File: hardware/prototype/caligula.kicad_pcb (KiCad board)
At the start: 2 copper layers, 89.8 x 108.2 mm, 105 parts, among them J1 USB2UART, J10 PT100_CONN, J2 1.47 IPS LCD, J3 ConnBattery, J4 USB2UART, J5 lcd jumper, J6 lcd jumper, J7 lcd jumper, J8 PH Sensor, Q1 SS8050, Q2 SS8050, Q3 SS8050, SW1 RST, SW2 IN1, SW3 Boot, SW4 IN2, SW5 IN4, SW6 IN4, SW7 MST22D18G2, U1 CH340C, U2 ESP32-S3-WROOM-1, U3 TPS63001_SEPIC_3V3, U4 ICL7660, U5 BQ24075RGT_DPPM, U6 ADS1115IDGS, U7 MAX31865xTP, U8 OPA2197xD

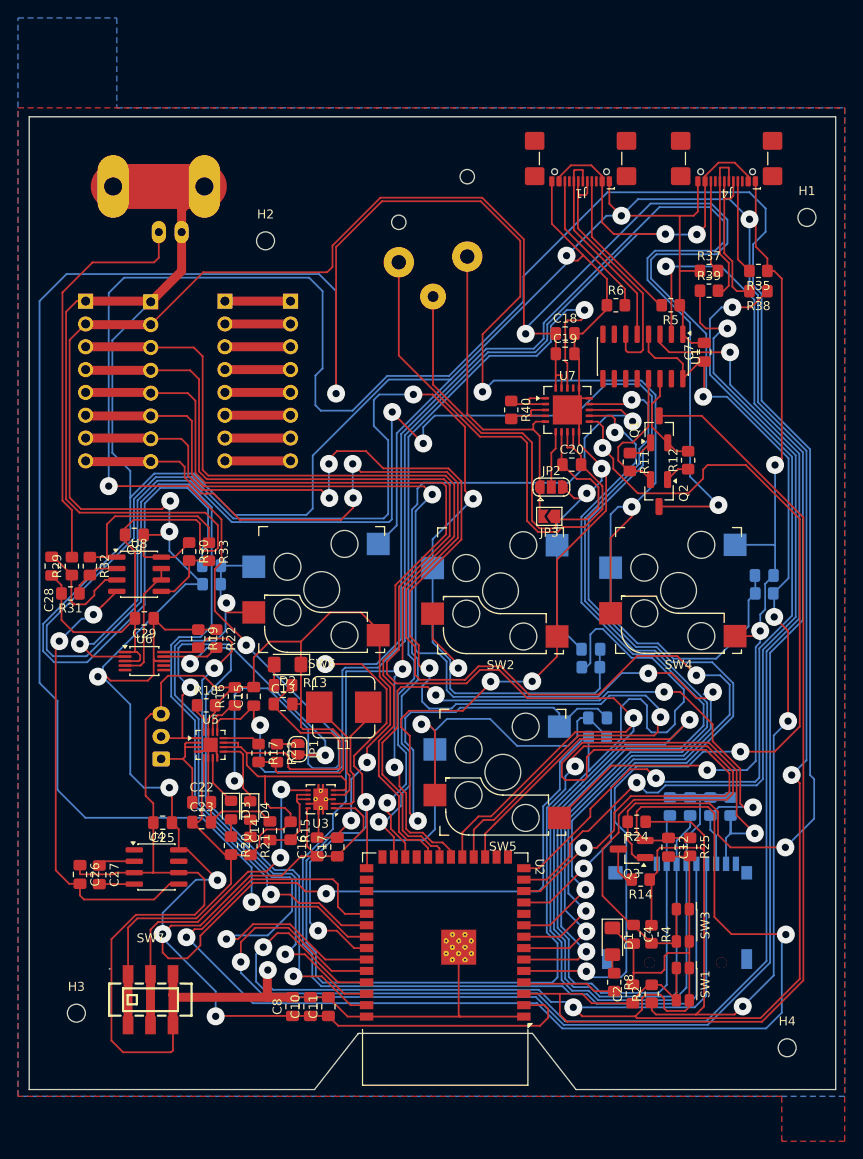
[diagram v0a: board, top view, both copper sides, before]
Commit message: feat: rechecking routing
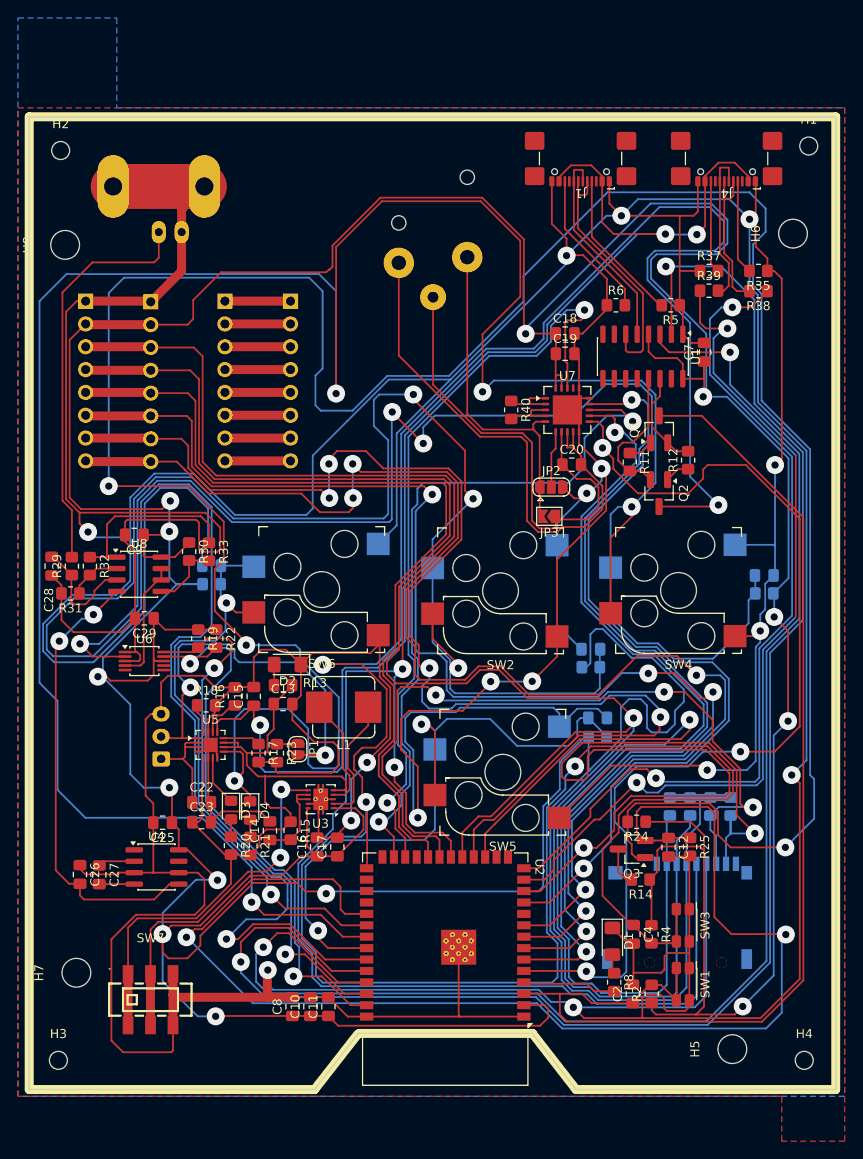
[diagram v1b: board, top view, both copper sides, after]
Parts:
- removed J10: PT100_CONN, Connector_Audio:Jack_XLR_Neutrik_NC3FAH1_Horizontal
- added H5: MountingHole, MountingHole:MountingHole_3.2mm_M3, F.Cu at (118.5, 146.8)
- added H6: MountingHole, MountingHole:MountingHole_3.2mm_M3, F.Cu at (125.2, 56.0)
- added H7: MountingHole, MountingHole:MountingHole_3.2mm_M3, F.Cu at (45.5, 138.2)
- added H8: MountingHole, MountingHole:MountingHole_3.2mm_M3, F.Cu at (44.2, 57.2)
- added J9: PT100_CONN, Connector_Audio:Jack_XLR_Neutrik_NC3FAH-0_Horizontal, B.Cu at (89.0, 58.6)
- moved H2 24.9 mm to (43.8, 46.8)
- moved H1 7.95 mm to (127.0, 46.2)
- moved H3 5.62 mm to (43.5, 148.0)
- moved H4 2.36 mm to (126.5, 148.0)
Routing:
- net GND: track 1104.7 -> 1084.6 mm, vias 16 -> 17
- net VDD: track 105.3 -> 89.3 mm
- net +3.3V: track 691.2 -> 697.1 mm
- net /TS: track 40.8 -> 44.6 mm
- net /IN1: track 236.5 -> 238.5 mm
- net /IN4: track 84.3 -> 82.5 mm
- net /BLK: track 158.2 -> 156.6 mm
- net /DC: track 147.9 -> 146.3 mm
- net /IO0: track 297.4 -> 298.7 mm
- net /I2C_SCL: track 61.4 -> 60.3 mm
- net /IN3: track 75.5 -> 76.4 mm
- net /MMC_CS: track 99.4 -> 100.1 mm
- net /I2C_SDA: track 65.1 -> 64.5 mm
- net /MISO: track 83.3 -> 83.9 mm
- net /CS: track 140.0 -> 139.5 mm
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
